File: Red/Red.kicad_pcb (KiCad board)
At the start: 4 copper layers, 44 x 67.5 mm, 82 parts, among them IC701 STM32G473CET6, J201 Conn_01x02, J301 Conn_01x03, J302 Screw_Terminal_01x02, J303 Screw_Terminal_01x02, J701 Conn_01x06, J801 USB_C_Receptacle, J802 Conn_01x10, J803 Conn_01x10, Q301 DMG3414U, Q302 DMG3414U, Q303 DMG3414U, Q304 DMG3414U, Q305 DMG3414U, SW701 SW_Push, U201 AZ1117-3.3, U202 AZ1117-5.0, U501 MPL115A1, U502 ICM-20948, U701 MAX7375AXR805, U801 FT230XS, Y701 SIT1533AI-H4-DCC-32.768E

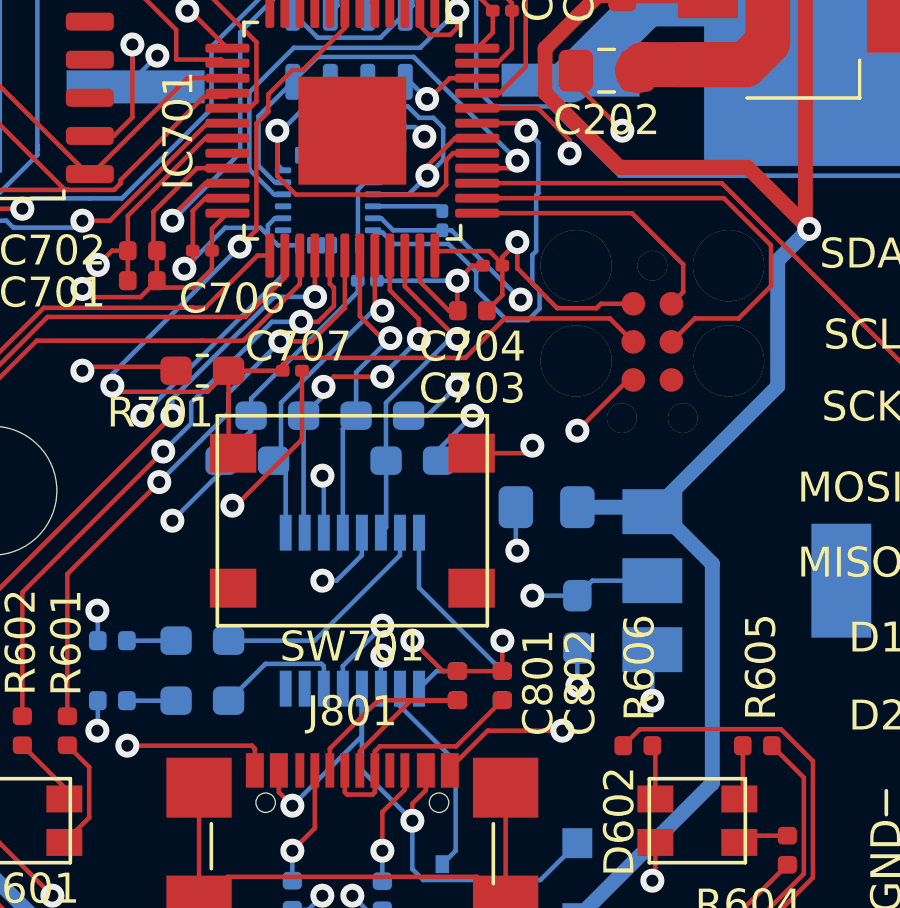
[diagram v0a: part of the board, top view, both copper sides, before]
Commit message: minor fixes
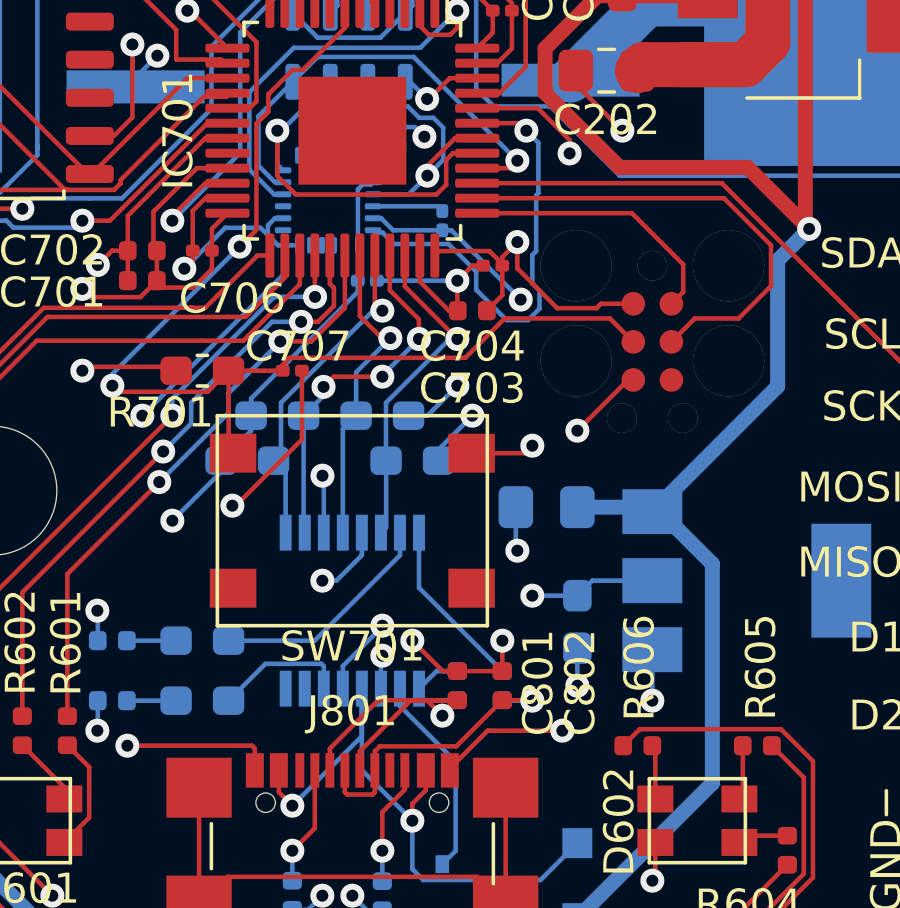
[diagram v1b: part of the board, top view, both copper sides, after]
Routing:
- net /IOConnector/USBD-: track 10.2 -> 12.9 mm, vias 0 -> 1
- net /IOConnector/USBD+: track 8.11 -> 10.1 mm, vias 0 -> 1
- net /IOConnector/MISO: track 46.6 -> 45.9 mm
